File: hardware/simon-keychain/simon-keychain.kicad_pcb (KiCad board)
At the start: 2 copper layers, 16 parts, among them SW1 SW_Push, SW2 SW_Push, SW3 SW_Push, SW4 SW_Push, U1 ATtiny85-20SU

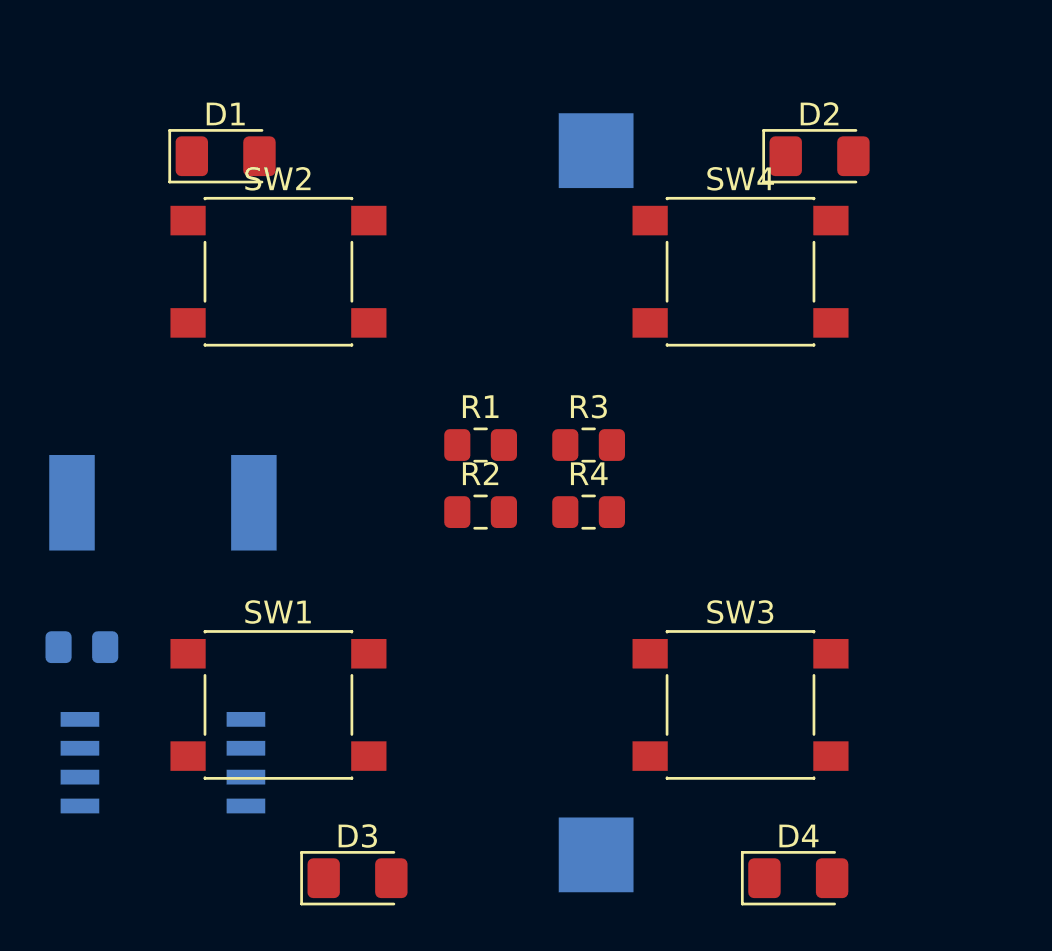
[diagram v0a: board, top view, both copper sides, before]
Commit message: update
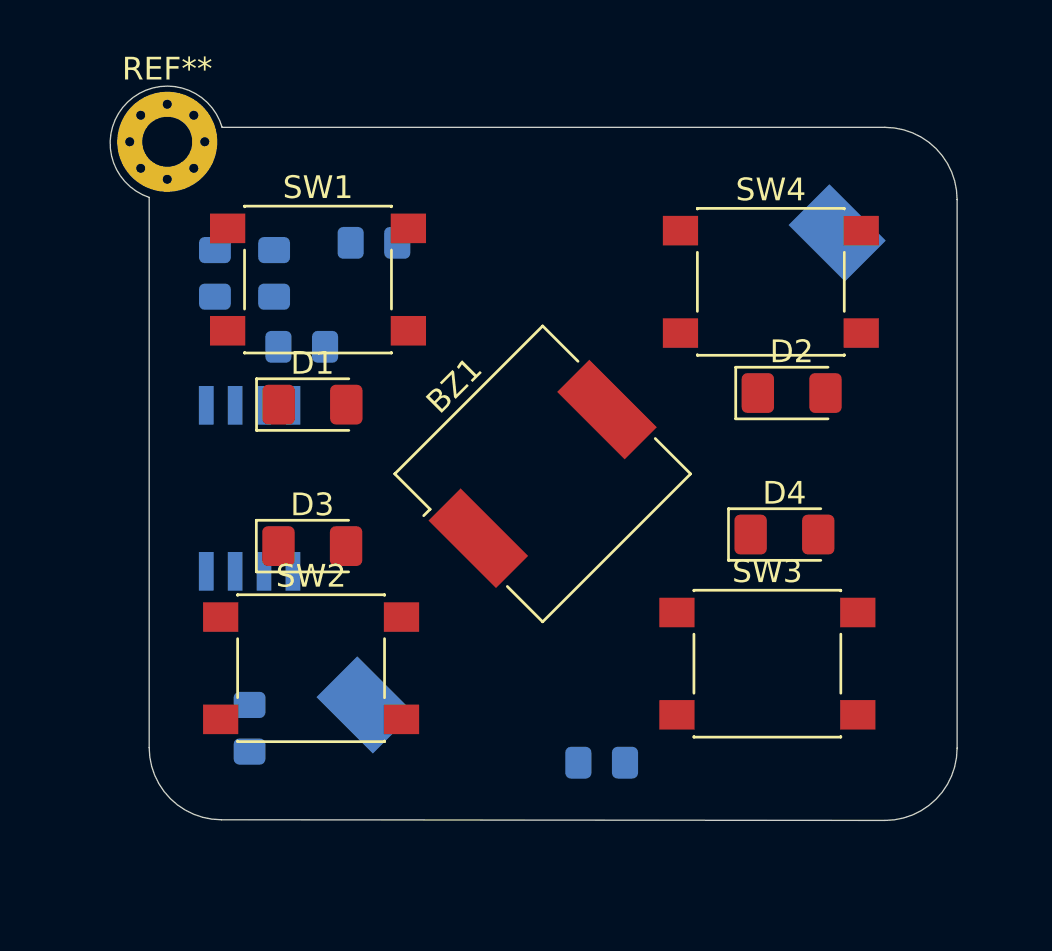
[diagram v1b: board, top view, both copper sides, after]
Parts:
- added C1: C, Capacitor_SMD:C_0805_2012Metric_Pad1.15x1.40mm_HandSolder, B.Cu at (142.0, 75.7)
- added REF**: MountingHole_2.2mm_M2_Pad_Via, MountingHole:MountingHole_2.2mm_M2_Pad_Via, F.Cu at (136.1, 66.7)
- BT1: footprint Batteries:BATT_CR2032_MPD -> Battery:BatteryHolder_Keystone_1058_1x2032
- BZ1: moved to F.Cu
- R1, R2, R3, R4: moved to B.Cu
- moved R3 19.4 mm to (139.7, 92.5), turned to 270 degrees
- moved SW1 18.8 mm to (142.7, 72.7)
- moved SW2 17.5 mm to (142.4, 89.8)
- moved R5 17.4 mm to (138.2, 72.5), turned to 270 degrees
- moved BZ1 16.7 mm to (152.6, 81.3), turned to 45 degrees
- moved R4 15.1 mm to (145.2, 71.1)
- moved D4 15.1 mm to (163.2, 83.9)
- moved D3 14.7 mm to (142.5, 84.5)
- moved U1 12.7 mm to (139.7, 81.9), turned to 90 degrees
- moved R2 12.2 mm to (155.2, 94.0)
- moved R1 11.8 mm to (140.8, 72.5), turned to 90 degrees
- moved D1 11.6 mm to (142.5, 78.2)
- moved D2 10.5 mm to (163.5, 77.7)
- moved SW3 2.16 mm to (162.5, 89.6)
- moved BT1 1.51 mm to (155.2, 81.1), turned to 45 degrees
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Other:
- board outline added: 37.2 x 32.3 mm

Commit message: PCB rooted
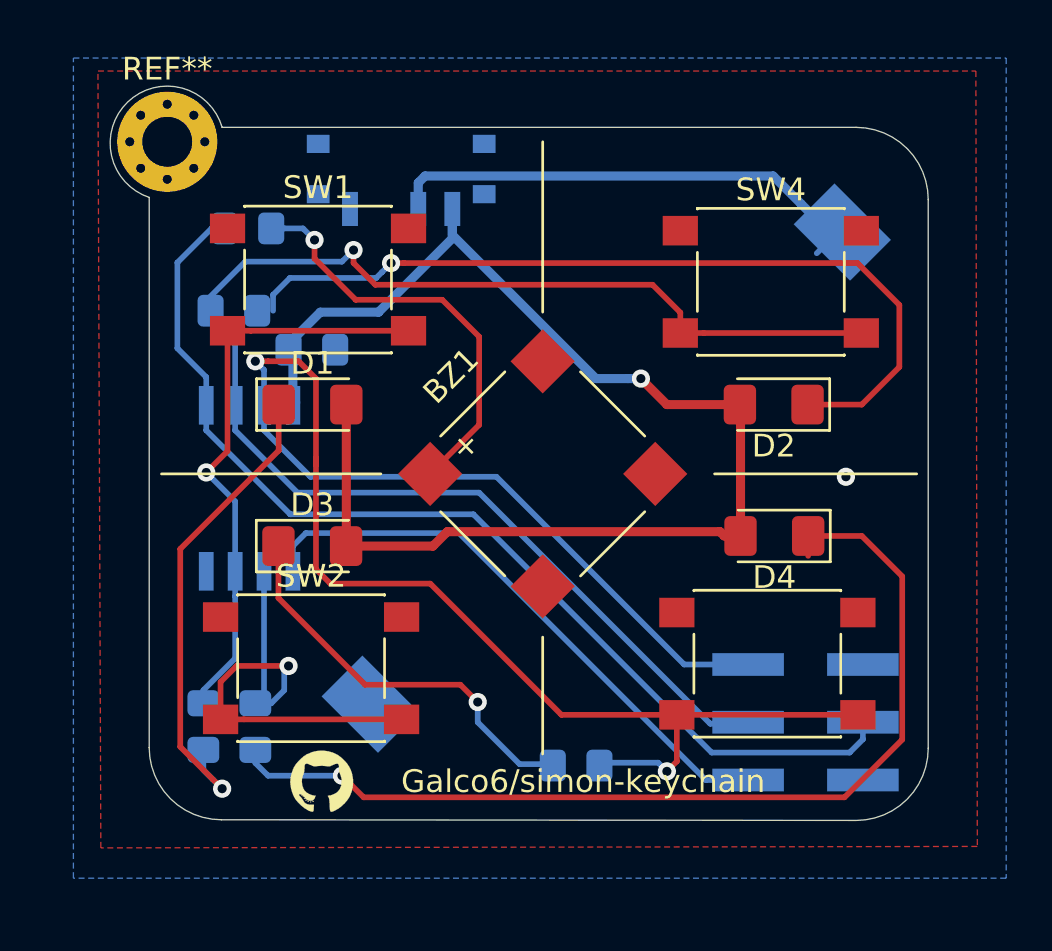
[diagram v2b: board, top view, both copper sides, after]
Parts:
- added G***: LOGO, Symbol:Github_logo, F.Cu at (142.9, 94.8)
- added J1: AVR-ISP-6, Connector_PinHeader_2.54mm:PinHeader_2x03_P2.54mm_Vertical_SMD_ISP, B.Cu at (164.1, 92.2)
- added SW5: SW_SPDT, Button_Switch_SMD:SW_SPDT_PCM12, B.Cu at (146.4, 68.2)
- BZ1: footprint Buzzer_Beeper:Buzzer_CUI_CPT-9019S-SMT -> Buzzer_Beeper:PUIAudio_SMT_0825_S_4_R
- SW1, SW2, SW3, SW4: footprint Button_Switch_SMD:SW_Push_1P1T_NO_6x6mm_H9.5mm -> Button_Switch_SMD:SW_SPST_PTS645
- moved R4 22.6 mm to (137.7, 92.4), turned to 90 degrees
- moved R5 2.45 mm to (139.6, 70.5), turned to 180 degrees
- moved R1 2.41 mm to (139.0, 74.1), turned to 180 degrees
- moved R2 1.13 mm to (154.1, 94.1)
- moved D2 0.94 mm to (162.8, 78.2), turned to 180 degrees
- moved C1 0.46 mm to (142.4, 75.8)
- moved D4 0.45 mm to (162.8, 84.0), turned to 180 degrees
- moved R3 0.26 mm to (140.0, 92.4), turned to 90 degrees
- moved BT1 0.23 mm to (155.4, 81.0), turned to 225 degrees
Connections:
- net Net-(R1-Pad2) renamed MISO
- net Net-(R2-Pad2) renamed SCK
- net Net-(R5-Pad2) renamed MOSI
- BT1 pad 1: +3V3 -> Net-(BT1-Pad1)
- U1 pad 1: Net-(U1-Pad1) -> RST
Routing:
- net SCK: track 0.00 -> 72.5 mm, vias 0 -> 2
- net MISO: track 0.00 -> 66.2 mm, vias 0 -> 1
- net +3V3: track 0.00 -> 59.6 mm, vias 0 -> 1
- net MOSI: track 0.00 -> 46.3 mm
- net Net-(D4-Pad1): track 0.00 -> 43.6 mm, vias 0 -> 1
- net Net-(D2-Pad1): track 0.00 -> 37.0 mm, vias 0 -> 1
- net RST: track 0.00 -> 25.9 mm
- net Net-(R4-Pad2): track 0.00 -> 25.8 mm, vias 0 -> 1
- net Net-(BT1-Pad1): track 0.00 -> 21.6 mm
- net Net-(R3-Pad2): track 0.00 -> 21.5 mm, vias 0 -> 1
- net Net-(D1-Pad1): track 0.00 -> 21.5 mm, vias 0 -> 1
- net Net-(BZ1-Pad1): track 0.00 -> 18.5 mm, vias 0 -> 1
- net Net-(D3-Pad1): track 0.00 -> 18.1 mm, vias 0 -> 1
- net GND: vias 0 -> 1
- added copper zone on B.Cu, net GND
- added copper zone on F.Cu, net GND
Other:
- board size 37.2 x 32.3 mm -> 36 x 32.3 mm
- board text added: "Galco6/simon-keychain"
